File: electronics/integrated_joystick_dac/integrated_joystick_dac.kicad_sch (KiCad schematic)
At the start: 11 parts, among them J1 Power/Signal Out, U1 raspberry_pi_pico, U2 MCP4728

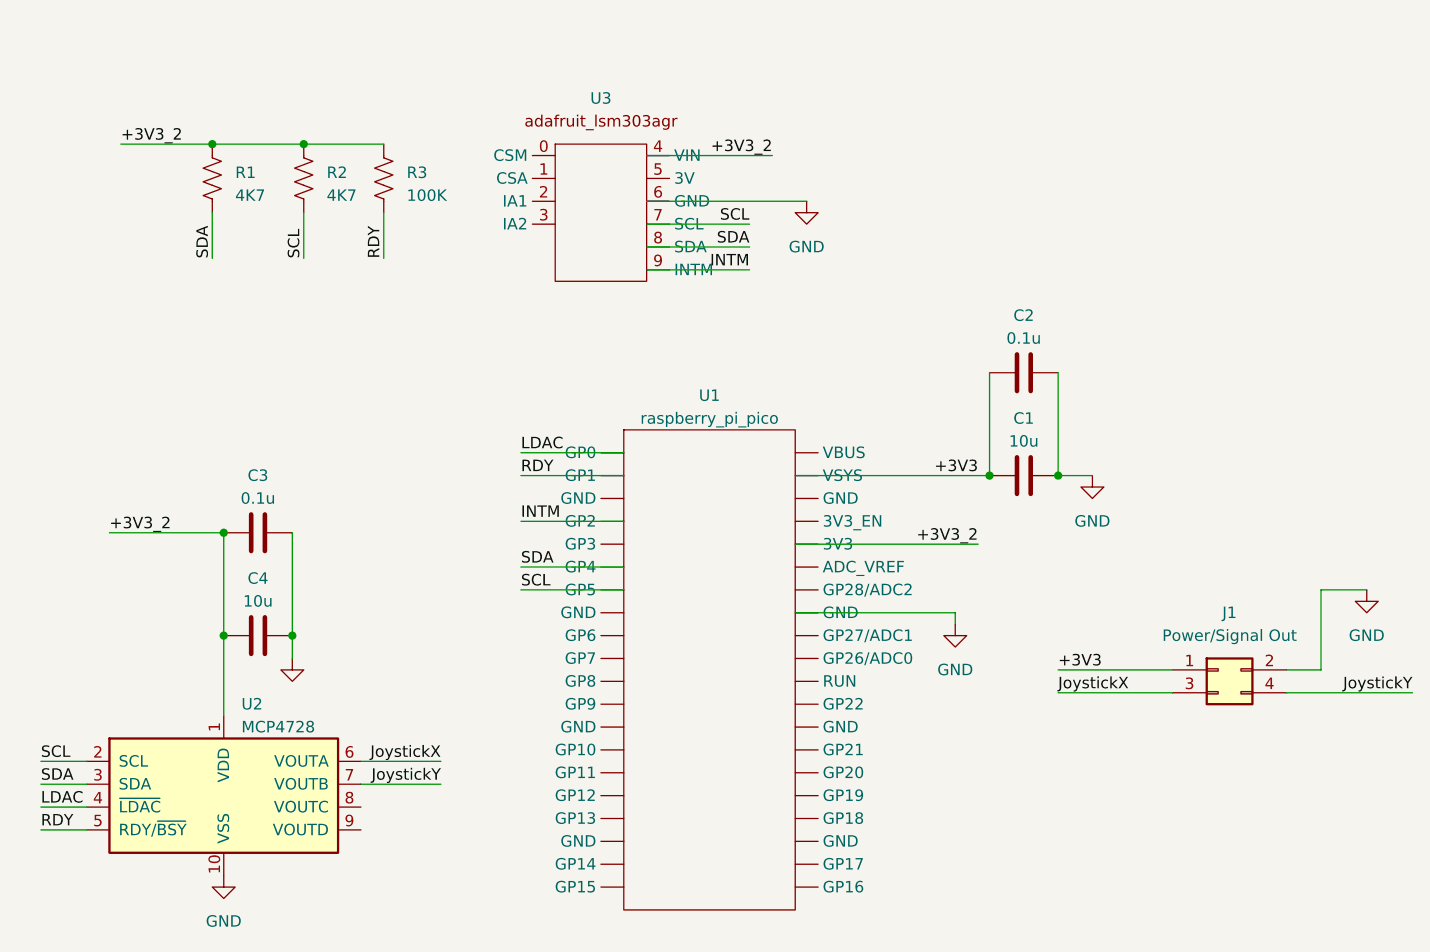
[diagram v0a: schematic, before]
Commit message: make smaller board...
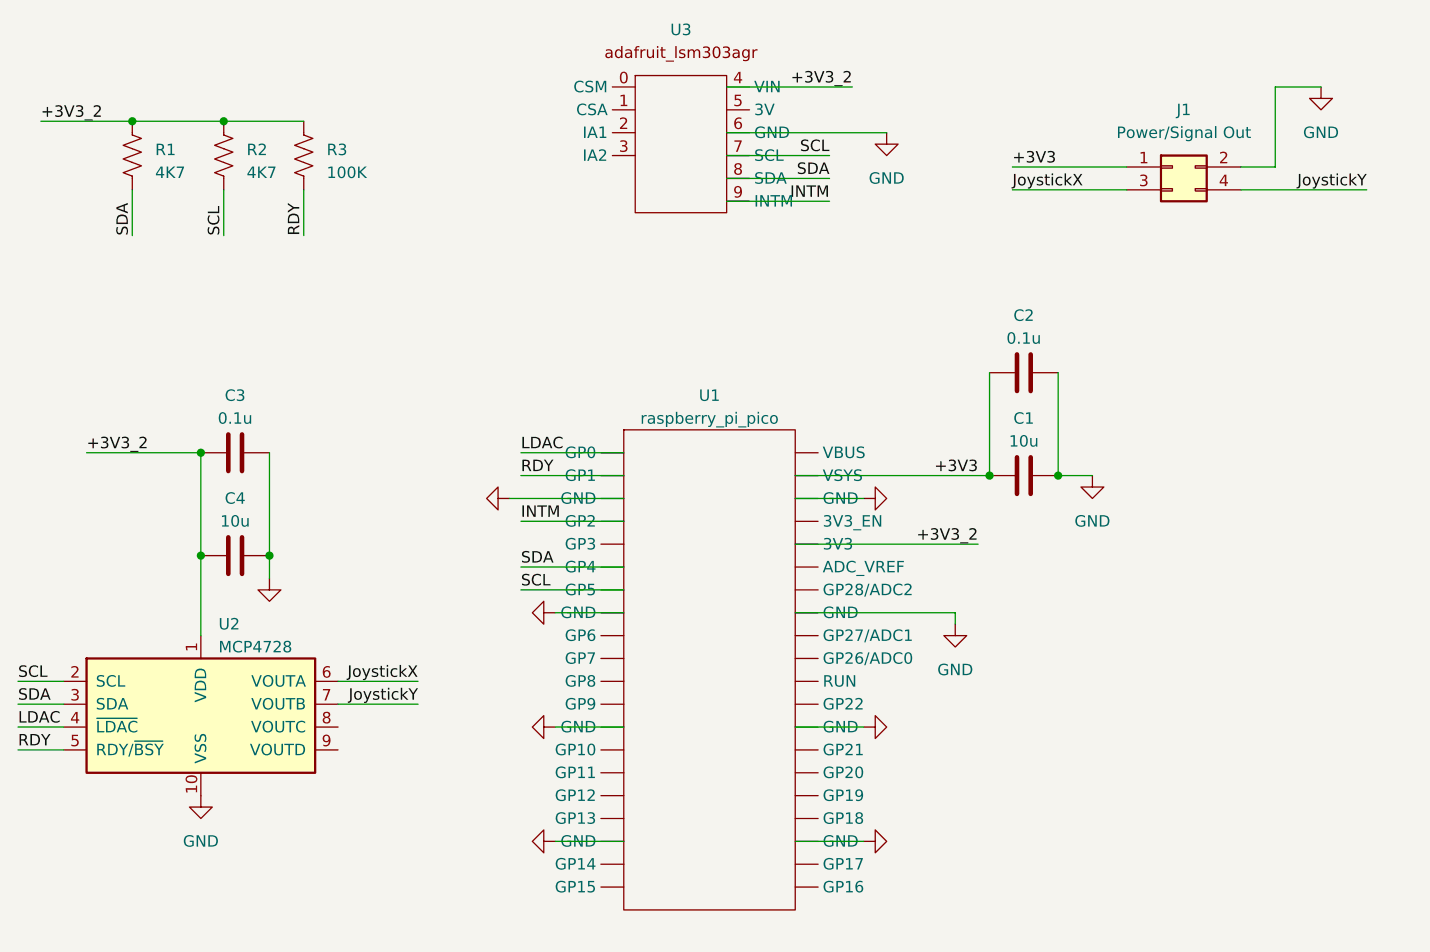
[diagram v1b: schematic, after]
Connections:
- net GND: now also U1.13 (GND), U1.18 (GND), U1.23 (GND), U1.28 (GND), U1.3 (GND), U1.38 (GND), U1.8 (GND)
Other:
- title: (none) -> Joystick DAC Board - Schematic
- moved on the sheet: C3, C4, J1, R1, R2, R3, U2, U3

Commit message: modify pcb and schematic sheets for export for design report
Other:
- company: (none) -> Sussex Tech Engineering
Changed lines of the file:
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@@
 (kicad_sch (version 20230121) (generator eeschema)
-  (paper "A4")
+  (paper "A")
   (title_block
     (title "Joystick DAC Board - Schematic")
+    (date "5/12/2023")
+    (rev "1")
+    (company "Sussex Tech Engineering")
   )
   (junction (at 133.35 76.2) (diameter 0) (color 0 0 0 0)
